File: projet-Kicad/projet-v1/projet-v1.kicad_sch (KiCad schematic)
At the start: 15 parts, among them J1 Power, J2 Digital/PWM, J3 Analog, J4 Digital/PWM

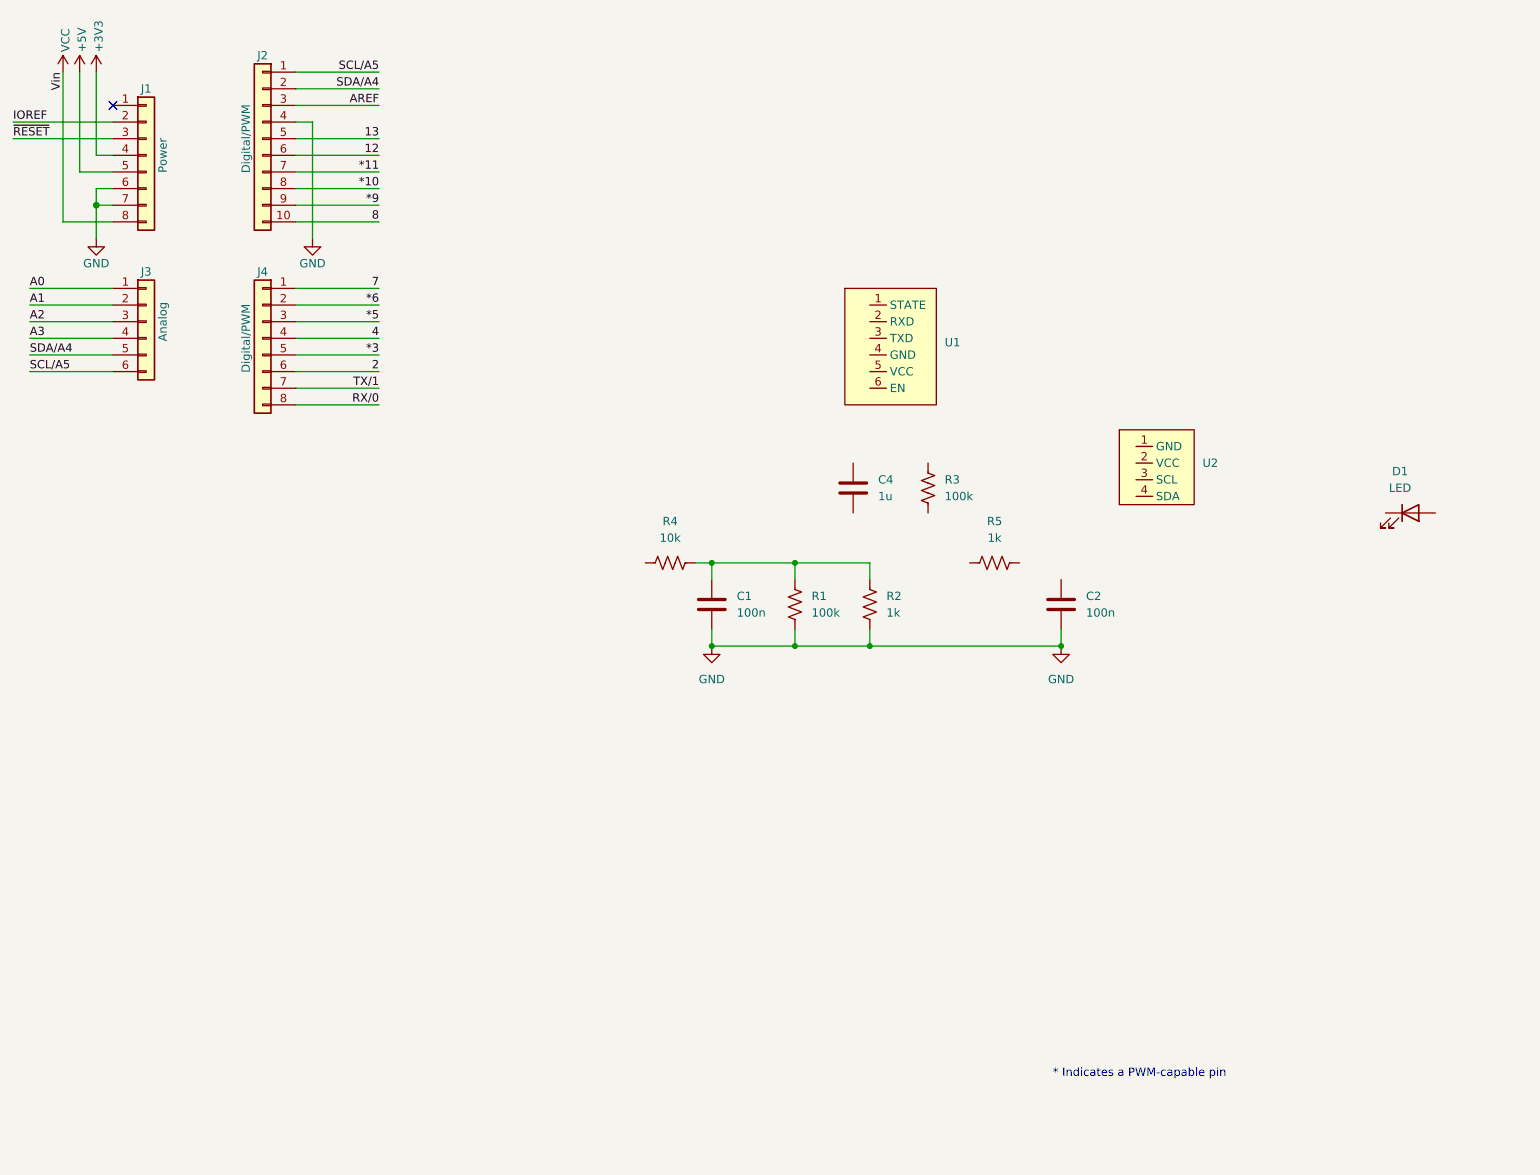
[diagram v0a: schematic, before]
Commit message: MAJ projet Kicad version envoyée à Cathy
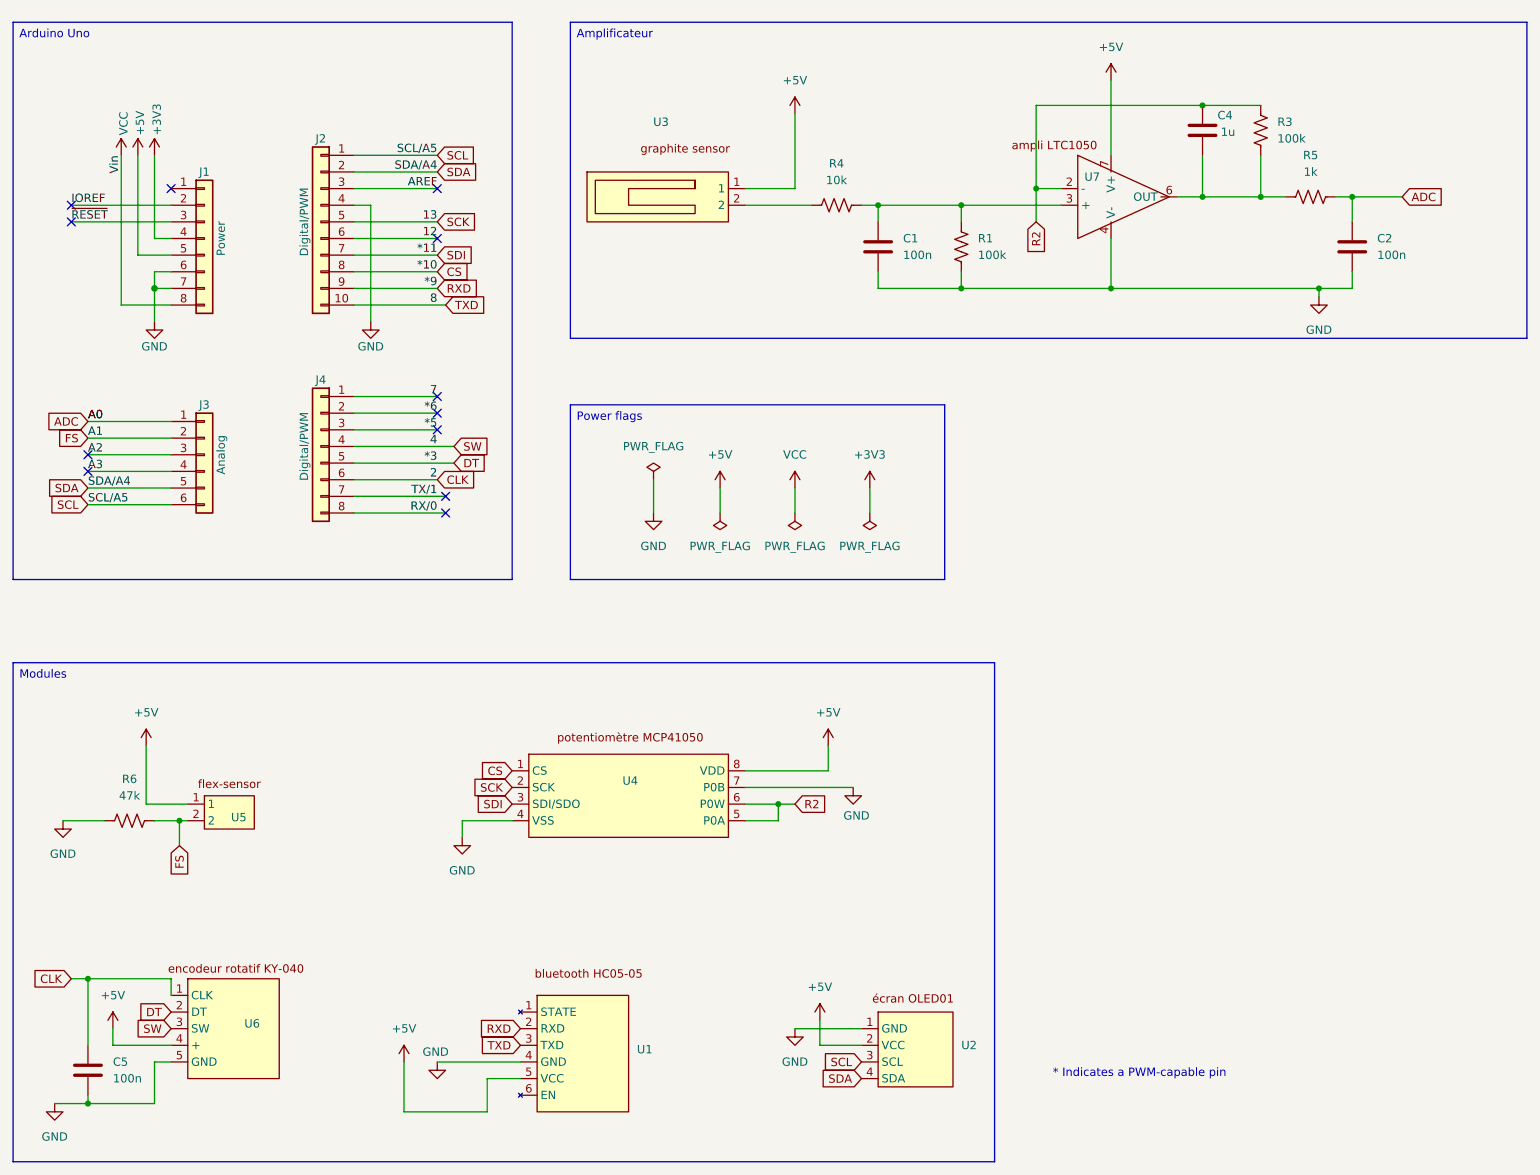
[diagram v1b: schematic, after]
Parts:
- removed D1: LED, LED_THT:LED_D3.0mm, symbol librairie-symboles:LED
- removed R2: 1k, Resistor_THT:R_Axial_DIN0207_L6.3mm_D2.5mm_P5.08mm_Vertical, symbol librairie-symboles:R_US
- added C5: 100n, Capacitor_THT:C_Disc_D4.7mm_W2.5mm_P5.00mm, symbol Device:C
- added R6: 47k, Resistor_THT:R_Axial_DIN0207_L6.3mm_D2.5mm_P5.08mm_Vertical, symbol librairie-symboles:R_US
- added U3: ~, librairie-empreintes:graphite-sensor, symbol librairie-symboles:graphite-sensor
- added U4: ~, librairie-empreintes:MCP41050, symbol librairie-symboles:MCP41050
- added U5: ~, librairie-empreintes:flex-sensor, symbol librairie-symboles:flex-sensor
- added U6: ~, librairie-empreintes:KY-040, symbol librairie-symboles:KY-040
- added U7: ~, librairie-empreintes:LTC1050, symbol librairie-symboles:LTC1050
- C1, C2: footprint Capacitor_THT:C_Disc_D3.0mm_W1.6mm_P2.50mm -> Capacitor_THT:C_Disc_D4.7mm_W2.5mm_P5.00mm
- C4: footprint Capacitor_THT:C_Disc_D3.0mm_W1.6mm_P2.50mm -> Capacitor_THT:C_Rect_L7.0mm_W4.5mm_P5.00mm
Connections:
- net *9 is gone; now on net RXD: J2.9 (Pin_9)
- net 8 is gone; now on net TXD: J2.10 (Pin_10)
- net A0 is gone; now on net ADC: J3.1 (Pin_1)
- net SCL/A5 is gone; now on net SCL: J2.1 (Pin_1), J3.6 (Pin_6)
- net SDA/A4 is gone; now on net SDA: J2.2 (Pin_2), J3.5 (Pin_5)
- net +5V: now also U1.5 (VCC), U2.2 (VCC), U3.1, U4.8 (VDD), U5.1, U6.4 (+), U7.7 (V+)
- net GND: now also U1.4 (GND), U2.1 (GND), C5.2, R6.1, U4.4 (VSS), U4.7 (P0B), U6.5 (GND), U7.4 (V-)
- net at C1.1, R1.1, R4.2: now also U7.3 (+)
- net SCL: now reaches U2.3 (SCL)
- net SDA: now reaches U2.4 (SDA)
- net R2: now reaches R3.1
- net R2: now also C4.1, U4.5 (P0A), U4.6 (P0W), U7.2 (-)
- net at R3.2: now also C4.2, R5.1, U7.6 (OUT)
- net at R4.1: now also U3.2
- net ADC: now reaches C2.1
- net ADC: now also R5.2
- net RXD: now reaches U1.2 (RXD)
- net TXD: now reaches U1.3 (TXD)
- net *10 renamed CS
- net CS: now also U4.1 (CS)
- net *11 renamed SDI
- net SDI: now also U4.3 (SDI/SDO)
- net *3 renamed DT
- net DT: now also U6.2 (DT)
- net 13 renamed SCK
- net SCK: now also U4.2 (SCK)
- net 2 renamed CLK
- net CLK: now also C5.1, U6.1 (CLK)
- net 4 renamed SW
- net SW: now also U6.3 (SW)
- net A1 renamed FS
- net FS: now also R6.2, U5.2
- no-connect marks 1 -> 12
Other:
- moved on the sheet: C1, C2, C4, J1, J2, J3, J4, R1, R3, R4, R5
